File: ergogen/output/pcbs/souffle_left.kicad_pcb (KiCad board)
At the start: 2 copper layers, 130 x 99.4 mm, 60 parts

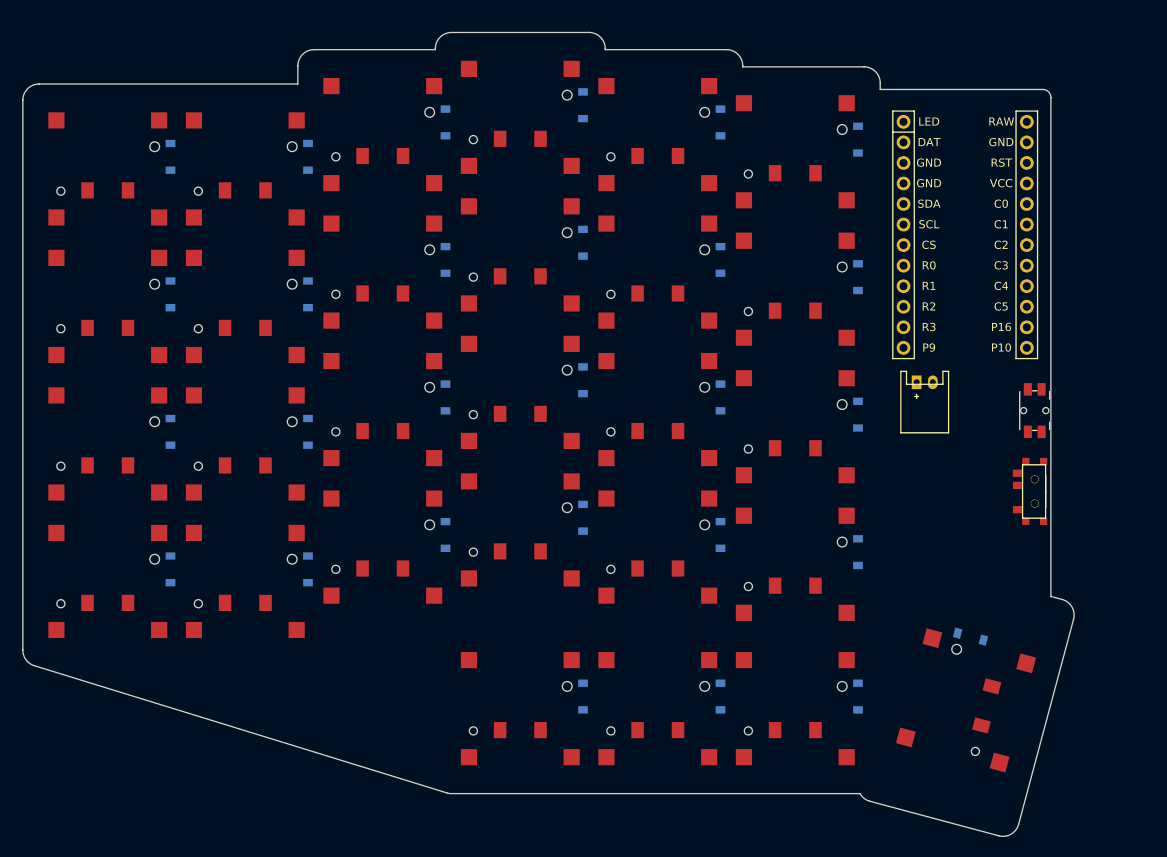
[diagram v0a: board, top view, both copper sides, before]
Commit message: feat: choc version
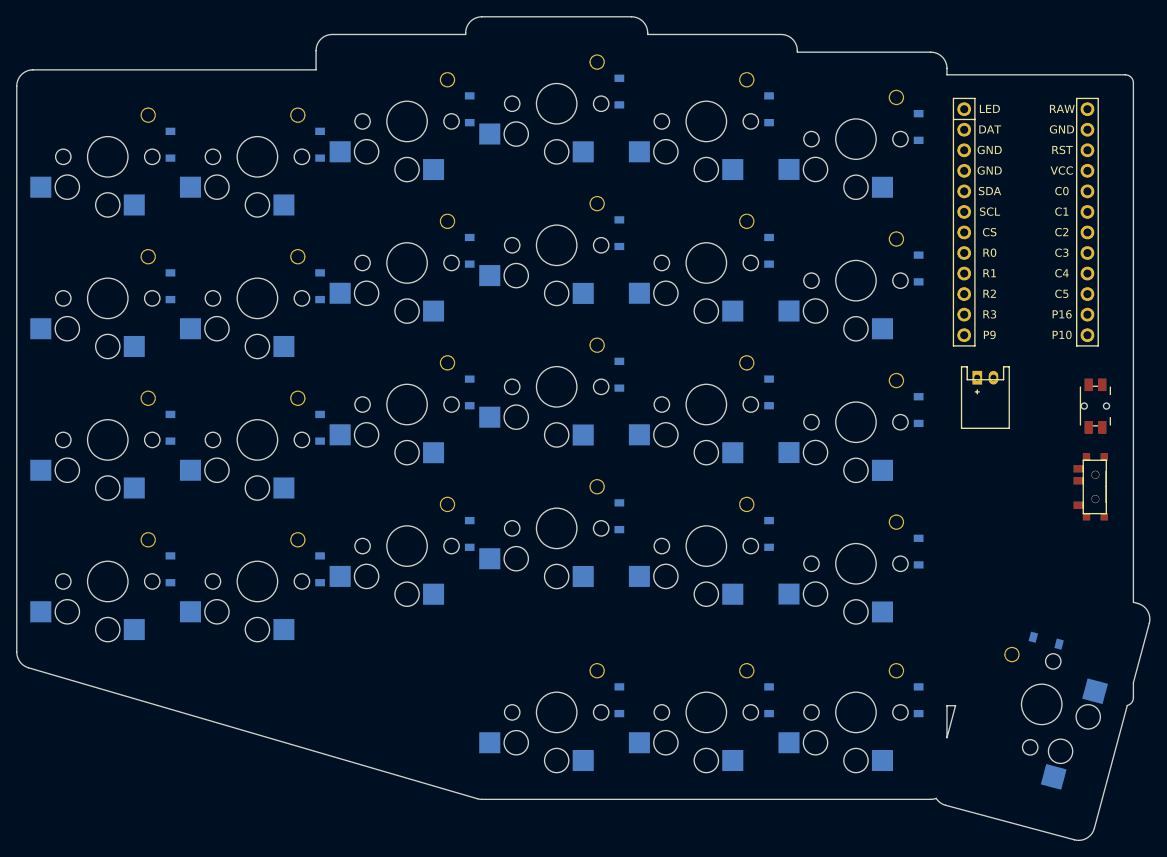
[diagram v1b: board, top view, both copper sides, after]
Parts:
- S1, S10, S11, S12, S13, S14, S15, S16, S17, S18, S19, S2, S20, S21, S22, S23, S24, S25, S26, S27, S28, S3, S4, S5, S6, S7, S8, S9: footprint CPG1316S01D02_mikeholscher -> ceoloide:switch_choc_v1_v2; moved to B.Cu
- moved D28 9.38 mm to (216.0, 107.3), turned to -15 degrees
- moved S28 9.38 mm to (215.5, 115.2), turned to 255 degrees
- moved D24 7.66 mm to (200.2, 43.8), turned to -90 degrees
- moved MCU1 7.66 mm to (213.5, 54.3)
- moved S24 7.66 mm to (192.5, 45.3), turned to 180 degrees
- moved D23 7.57 mm to (200.2, 61.3), turned to -90 degrees
- moved S23 7.57 mm to (192.5, 62.8), turned to 180 degrees
- moved B1 7.52 mm to (222.1, 78.3)
- moved D22 7.52 mm to (200.2, 78.8), turned to -90 degrees
- moved JST1 7.52 mm to (208.5, 74.8)
- moved S22 7.52 mm to (192.5, 80.3), turned to 180 degrees
- moved T1 7.52 mm to (222.1, 88.3)
- moved D27 7.51 mm to (200.2, 114.7), turned to -90 degrees
- moved S27 7.51 mm to (192.5, 116.2), turned to 180 degrees
- moved D21 7.50 mm to (200.2, 96.3), turned to -90 degrees
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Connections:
- S1 pad 1: outer_bottom -> C0
- S1 pad 2: C0 -> outer_bottom
- S10 pad 1: ring_home -> C2
- S10 pad 2: C2 -> ring_home
- S11 pad 1: ring_top -> C2
- S11 pad 2: C2 -> ring_top
- S12 pad 1: ring_number -> C2
- S12 pad 2: C2 -> ring_number
- S13 pad 1: middle_bottom -> C3
- S13 pad 2: C3 -> middle_bottom
- S14 pad 1: middle_home -> C3
- S14 pad 2: C3 -> middle_home
- S15 pad 1: middle_top -> C3
- S15 pad 2: C3 -> middle_top
- S16 pad 1: middle_number -> C3
- S16 pad 2: C3 -> middle_number
- S17 pad 1: index_bottom -> C4
- S17 pad 2: C4 -> index_bottom
- S18 pad 1: index_home -> C4
- S18 pad 2: C4 -> index_home
- S19 pad 1: index_top -> C4
- S19 pad 2: C4 -> index_top
- S2 pad 1: outer_home -> C0
- S2 pad 2: C0 -> outer_home
- S20 pad 1: index_number -> C4
- S20 pad 2: C4 -> index_number
- S21 pad 1: inner_bottom -> C5
- S21 pad 2: C5 -> inner_bottom
- S22 pad 1: inner_home -> C5
- S22 pad 2: C5 -> inner_home
- S23 pad 1: inner_top -> C5
- S23 pad 2: C5 -> inner_top
- S24 pad 1: inner_number -> C5
- S24 pad 2: C5 -> inner_number
- S25 pad 1: inward_home -> C2
- S25 pad 2: C2 -> inward_home
- S26 pad 1: outward_home -> C3
- S26 pad 2: C3 -> outward_home
- S27 pad 1: small_thumbkey_home -> C4
- S27 pad 2: C4 -> small_thumbkey_home
- S28 pad 1: thumbkey_home -> C5
- S28 pad 2: C5 -> thumbkey_home
- S3 pad 1: outer_top -> C0
- S3 pad 2: C0 -> outer_top
- S4 pad 1: outer_number -> C0
- S4 pad 2: C0 -> outer_number
- S5 pad 1: pinky_bottom -> C1
- S5 pad 2: C1 -> pinky_bottom
- S6 pad 1: pinky_home -> C1
- S6 pad 2: C1 -> pinky_home
- S7 pad 1: pinky_top -> C1
- S7 pad 2: C1 -> pinky_top
- S8 pad 1: pinky_number -> C1
- S8 pad 2: C1 -> pinky_number
- S9 pad 1: ring_bottom -> C2
- S9 pad 2: C2 -> ring_bottom
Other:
- board size 130 x 99.4 mm -> 140.1 x 101.8 mm
